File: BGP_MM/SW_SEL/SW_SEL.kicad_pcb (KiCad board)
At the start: 2 copper layers, 15 x 15 mm, 3 parts, among them J1 CONN_01X03, J2 Conn_01x02_Male, SW1 Switch_SPDT_x2

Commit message: MM Refactoring
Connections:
- net /SIG_O renamed /SEL_O
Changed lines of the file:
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@@
     (links 7)
     (no_connects 0)
-    (area 136.924999 82.924999 154.075001 98.075001)
+    (area 136.924999 82.924999 152.075001 98.075001)
     (thickness 1.6)
     (drawings 5)
@@
   (net 0 "")
   (net 1 Earth)
-  (net 2 /SIG_O)
-  (net 3 /I_BR)
-  (net 4 /I_NK)
+  (net 2 /I_BR)
+  (net 3 /I_NK)
+  (net 4 /SEL_O)
   (net_class Default "This is the default net class."
     (clearance 0.3)
@@
     (add_net /I_BR)
     (add_net /I_NK)
-    (add_net /SIG_O)
+    (add_net /SEL_O)
     (add_net Earth)
   )
@@
     (fp_line (start 1.65 3.3) (end 1.65 -8.1) (layer F.SilkS) (width 0.15))
     (pad 5 thru_hole oval (at -4.7 -4.8 270) (size 1.8 1.8) (drill 1) (layers *.Cu *.Mask)
-      (net 4 /I_NK))
+      (net 3 /I_NK))
     (pad 4 thru_hole circle (at 0 -4.8 270) (size 1.8 1.8) (drill 1) (layers *.Cu *.Mask)
-      (net 2 /SIG_O))
+      (net 4 /SEL_O))
     (pad 6 thru_hole oval (at -9.4 -4.8 270) (size 1.8 1.8) (drill 1) (layers *.Cu *.Mask)
       (net 1 Earth))
@@
       (net 1 Earth))
     (pad 2 thru_hole oval (at -4.7 0.03 270) (size 1.8 1.8) (drill 1) (layers *.Cu *.Mask)
-      (net 3 /I_BR))
+      (net 2 /I_BR))
     (pad 3 thru_hole oval (at -9.4 0.03 270) (size 1.8 1.8) (drill 1) (layers *.Cu *.Mask)
-      (net 2 /SIG_O))
+      (net 4 /SEL_O))
     (model ${KISYS3DMOD}/TerminalBlock_Phoenix.3dshapes/TerminalBlock_Phoenix_MPT-2.54mm_2pol.wrl
       (at (xyz 0.05 0 0))
@@
       (net 1 Earth))
     (pad 2 thru_hole oval (at 2 0 90) (size 1.2 1.7) (drill 0.75) (layers *.Cu *.Mask)
-      (net 3 /I_BR))
+      (net 2 /I_BR))
     (pad 3 thru_hole oval (at 4 0 90) (size 1.2 1.7) (drill 0.75) (layers *.Cu *.Mask)
-      (net 4 /I_NK))
+      (net 3 /I_NK))
     (model ${KISYS3DMOD}/Connectors_JST.3dshapes/JST_PH_B3B-PH-K_03x2.00mm_Straight.wrl
       (at (xyz 0 0 0))
@@
       (net 1 Earth))
     (pad 2 thru_hole oval (at 2 0 90) (size 1.2 1.7) (drill 0.75) (layers *.Cu *.Mask)
-      (net 2 /SIG_O))
+      (net 4 /SEL_O))
     (model ${KISYS3DMOD}/Connectors_JST.3dshapes/JST_PH_B2B-PH-K_02x2.00mm_Straight.wrl
       (at (xyz 0 0 0))
@@
   (gr_line (start 137 83) (end 152 83) (layer Edge.Cuts) (width 0.15))
   (gr_line (start 137 98) (end 137 83) (layer Edge.Cuts) (width 0.15))
-  (segment (start 145.23 95.2) (end 142.8 92.77) (width 0.5) (layer B.Cu) (net 2))
-  (segment (start 142.8 92.77) (end 142.8 88.2) (width 0.5) (layer B.Cu) (net 2))
-  (segment (start 142.8 88.2) (end 141.299999 86.699999) (width 0.5) (layer B.Cu) (net 2))
-  (segment (start 141.299999 86.699999) (end 140.4 85.8) (width 0.5) (layer B.Cu) (net 2))
-  (segment (start 149.8 93.6) (end 146.83 93.6) (width 0.5) (layer B.Cu) (net 2))
-  (segment (start 146.83 93.6) (end 145.23 95.2) (width 0.5) (layer B.Cu) (net 2))
-  (segment (start 149.8 87.1) (end 148.63 87.1) (width 0.5) (layer F.Cu) (net 3))
-  (segment (start 148.63 87.1) (end 146.129999 89.600001) (width 0.5) (layer F.Cu) (net 3))
-  (segment (start 146.129999 89.600001) (end 145.23 90.5) (width 0.5) (layer F.Cu) (net 3))
-  (segment (start 149.8 85.1) (end 148.45 85.1) (width 0.5) (layer F.Cu) (net 4))
-  (segment (start 148.45 85.1) (end 143.05 90.5) (width 0.5) (layer F.Cu) (net 4))
-  (segment (start 143.05 90.5) (end 141.672792 90.5) (width 0.5) (layer F.Cu) (net 4))
-  (segment (start 141.672792 90.5) (end 140.4 90.5) (width 0.5) (layer F.Cu) (net 4))
+  (segment (start 149.8 87.1) (end 148.63 87.1) (width 0.5) (layer F.Cu) (net 2))
+  (segment (start 148.63 87.1) (end 146.129999 89.600001) (width 0.5) (layer F.Cu) (net 2))
+  (segment (start 146.129999 89.600001) (end 145.23 90.5) (width 0.5) (layer F.Cu) (net 2))
+  (segment (start 149.8 85.1) (end 148.45 85.1) (width 0.5) (layer F.Cu) (net 3))
+  (segment (start 148.45 85.1) (end 143.05 90.5) (width 0.5) (layer F.Cu) (net 3))
+  (segment (start 143.05 90.5) (end 141.672792 90.5) (width 0.5) (layer F.Cu) (net 3))
+  (segment (start 141.672792 90.5) (end 140.4 90.5) (width 0.5) (layer F.Cu) (net 3))
+  (segment (start 145.23 95.2) (end 142.8 92.77) (width 0.5) (layer B.Cu) (net 4))
+  (segment (start 142.8 92.77) (end 142.8 88.2) (width 0.5) (layer B.Cu) (net 4))
+  (segment (start 142.8 88.2) (end 141.299999 86.699999) (width 0.5) (layer B.Cu) (net 4))
+  (segment (start 141.299999 86.699999) (end 140.4 85.8) (width 0.5) (layer B.Cu) (net 4))
+  (segment (start 149.8 93.6) (end 146.83 93.6) (width 0.5) (layer B.Cu) (net 4))
+  (segment (start 146.83 93.6) (end 145.23 95.2) (width 0.5) (layer B.Cu) (net 4))
   (zone (net 1) (net_name Earth) (layer F.Cu) (hatch edge 0.508)
     (connect_pads (clearance 0.3))

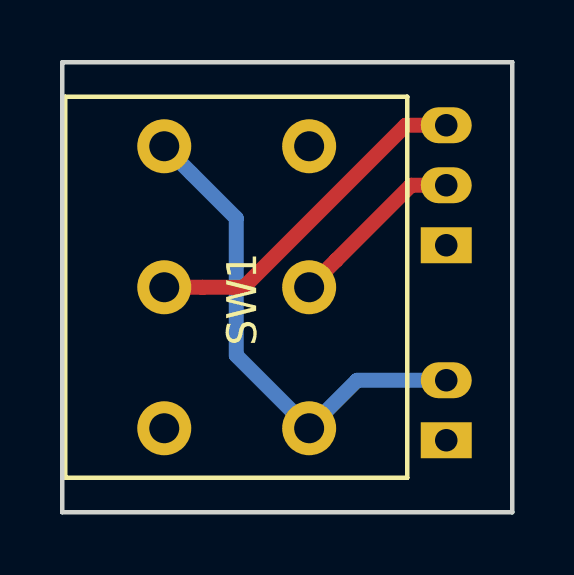
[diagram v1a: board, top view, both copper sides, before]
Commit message: MM Refactoring
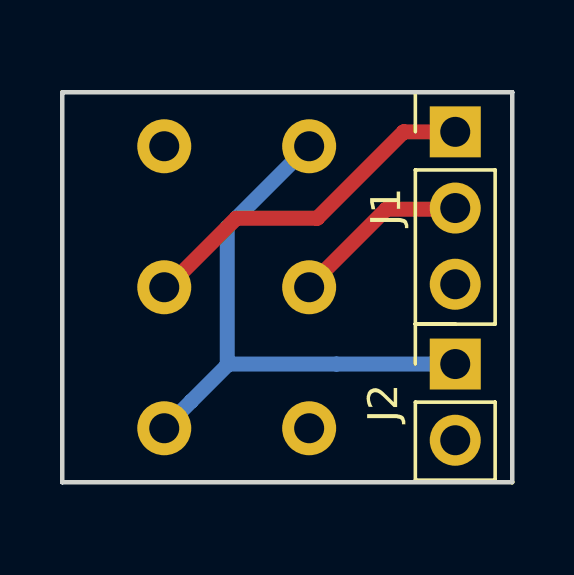
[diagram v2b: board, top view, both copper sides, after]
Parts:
- J1: value CONN_01X03 -> Conn_01x03_Male; footprint Connectors_JST:JST_PH_B3B-PH-K_03x2.00mm_Straight -> Pin_Headers:Pin_Header_Straight_1x03_Pitch2.54mm; moved to F.Cu
- J2: footprint Connectors_JST:JST_PH_B2B-PH-K_02x2.00mm_Straight -> Pin_Headers:Pin_Header_Straight_1x02_Pitch2.54mm; moved to F.Cu
- SW1: moved to B.Cu
- moved SW1 9.40 mm to (145.2, 95.2), turned to 270 degrees
- moved J1 3.79 mm to (150.1, 85.3), turned to 0 degrees
- moved J2 2.56 mm to (150.1, 93.1), turned to 0 degrees
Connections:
- J1 pad 1: Earth -> /I_NK
- J1 pad 3: /I_NK -> Earth
- J2 pad 1: Earth -> /SEL_O
- J2 pad 2: /SEL_O -> Earth
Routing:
- net /SEL_O: track 16.6 -> 19.0 mm
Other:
- board size 15 x 15 mm -> 15 x 13 mm
- board text removed: "MM Sabre Sel Switch"
